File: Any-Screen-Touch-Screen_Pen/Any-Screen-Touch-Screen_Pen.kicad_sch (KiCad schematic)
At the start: 51 parts, among them J1 PEN_BUTTON, J2 Reset button, J3 Flash button, J4 Battery Terminals, J5 Power Switch, J6 LED1, J7 LED2, J8 LED3, J9 LED4, P1 USB_C_Plug_USB2.0, Q1 S8050, Q2 S8050, Q3 IRLZ44N, U1 CP2104, U2 ESP32-S3-WROOM-1, U3 BQ27441-G1, U4 LSM6DSL, U5 AMS1117-1.8

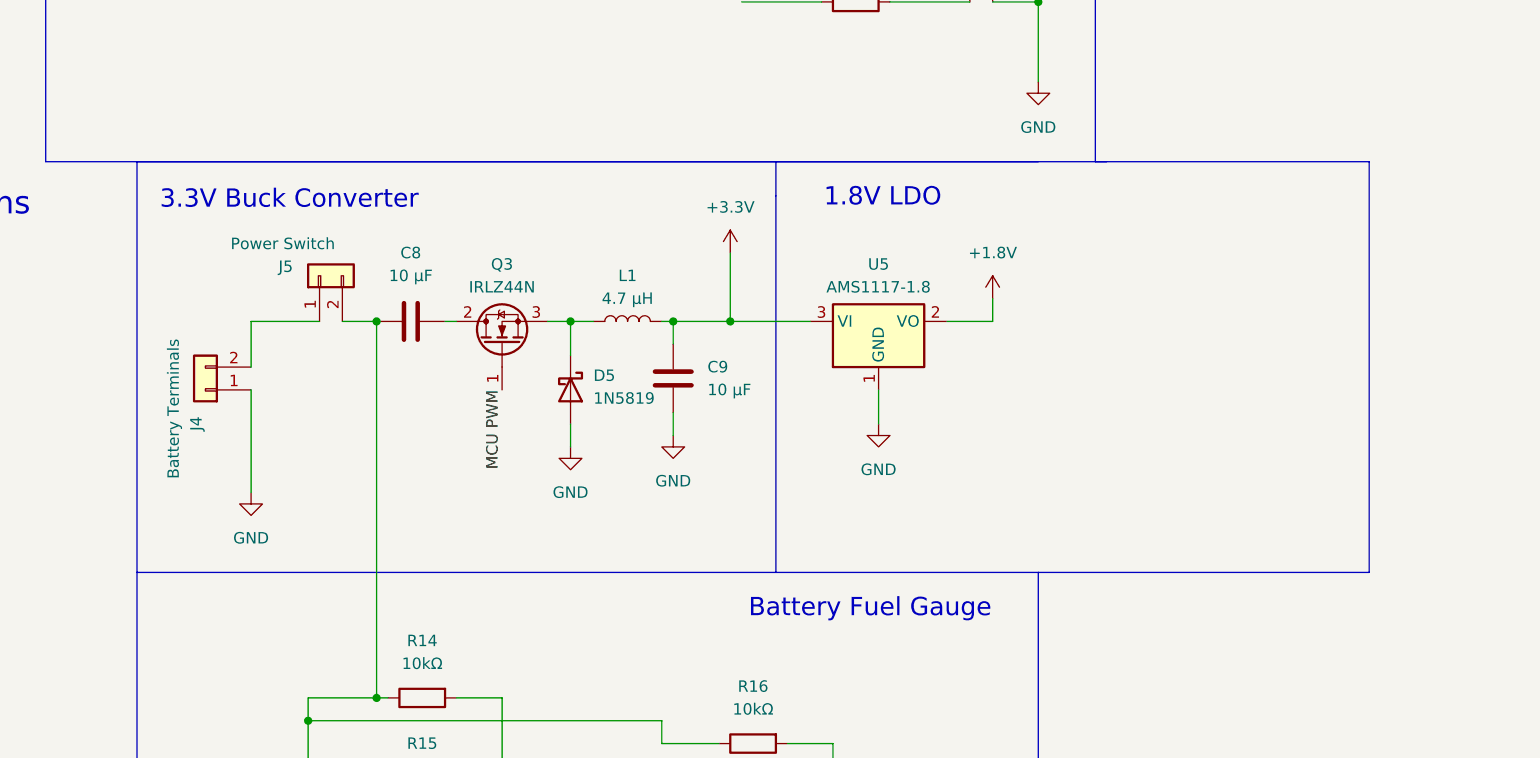
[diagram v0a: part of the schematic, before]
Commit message: Started PCB layout and organized components
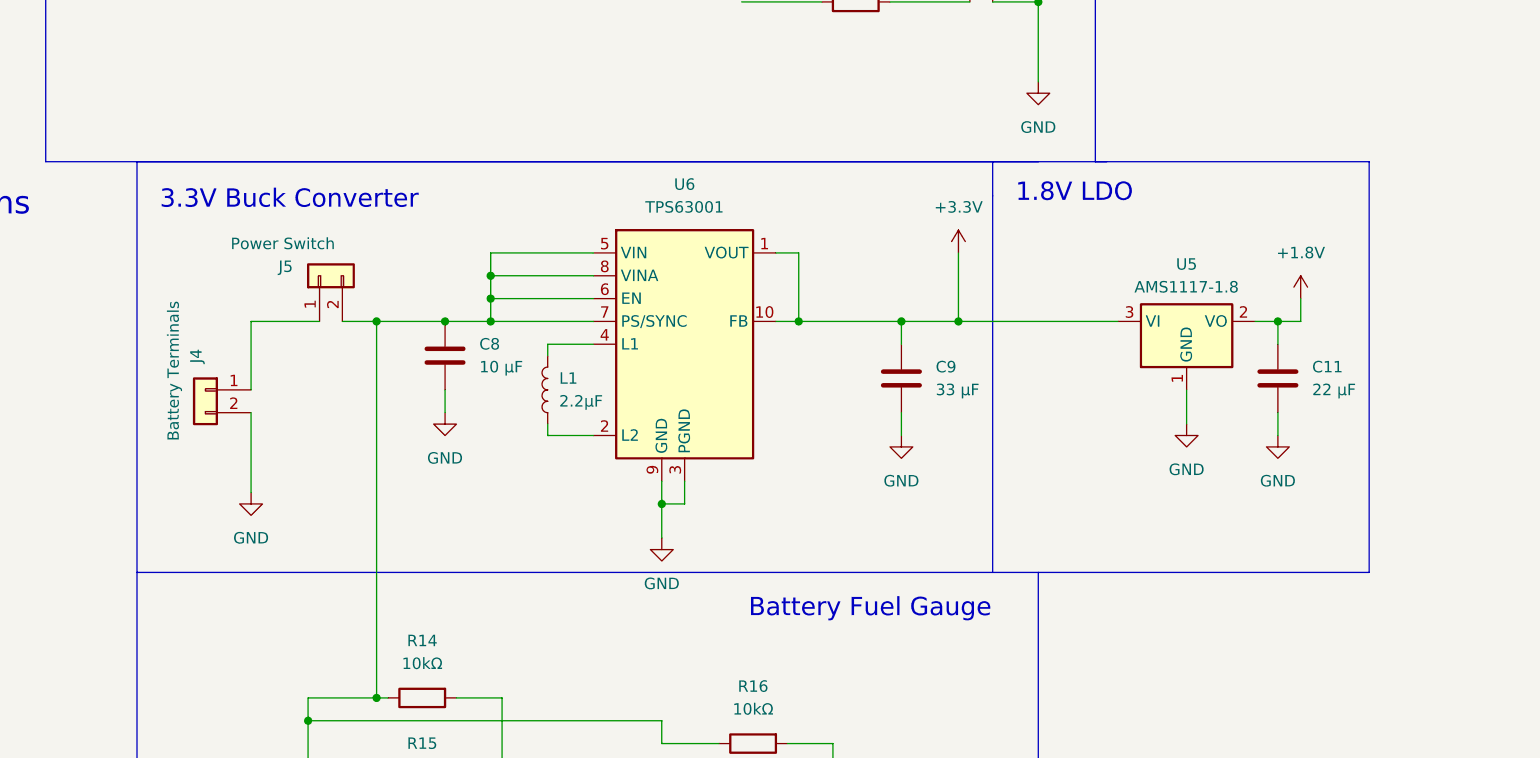
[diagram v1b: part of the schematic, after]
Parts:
- removed D5: 1N5819, Diode_THT:D_DO-41_SOD81_P10.16mm_Horizontal, symbol Diode:1N5819
- removed Q3: IRLZ44N, Package_TO_SOT_THT:TO-220-3_Vertical, symbol Transistor_FET:IRLZ44N
- added C11: 22 μF, Capacitor_SMD:C_0805_2012Metric_Pad1.18x1.45mm_HandSolder, symbol Device:C
- added U6: TPS63001, Package_SON:Texas_DRC0010J_ThermalVias, symbol Regulator_Switching:TPS63001
- C8: footprint (none) -> Capacitor_SMD:C_0805_2012Metric_Pad1.18x1.45mm_HandSolder
- C9: value 10 μF -> 33 μF; footprint (none) -> Capacitor_SMD:C_0805_2012Metric_Pad1.18x1.45mm_HandSolder
- L1: value 4.7 μH -> 2.2μF
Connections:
- net +1.8V: now also C11.1
- net +3.3V: now also U6.1 (VOUT), U6.10 (FB); no longer L1.2
- net GND: now also C8.1, J4.2 (Pin_2), C11.2, U6.11 (PGND), U6.3 (PGND), U6.9 (GND); no longer J4.1 (Pin_1)
- net at L1.1: now also U6.2 (L2)
- net at J5.1 (Pin_1): now also J4.1 (Pin_1); no longer J4.2 (Pin_2)
- net at C7.1, C8.2, J5.2 (Pin_2)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: now also U6.5 (VIN), U6.6 (EN), U6.7 (PS/SYNC), U6.8 (VINA)
- new net: L1.2, U6.4 (L1)
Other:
- moved on the sheet: U5
